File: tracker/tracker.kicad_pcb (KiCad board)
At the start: 2 copper layers, 26 parts, among them J1 USB_C_Receptacle_PowerOnly_6P, Q1 DMG9926UDM-7, U1 XIAO-ESP32-C6-SMD, U2 LIS3DH, U3 DW01A, U4 INA226AIDGSR, U5 TP4056-42-ESOP8

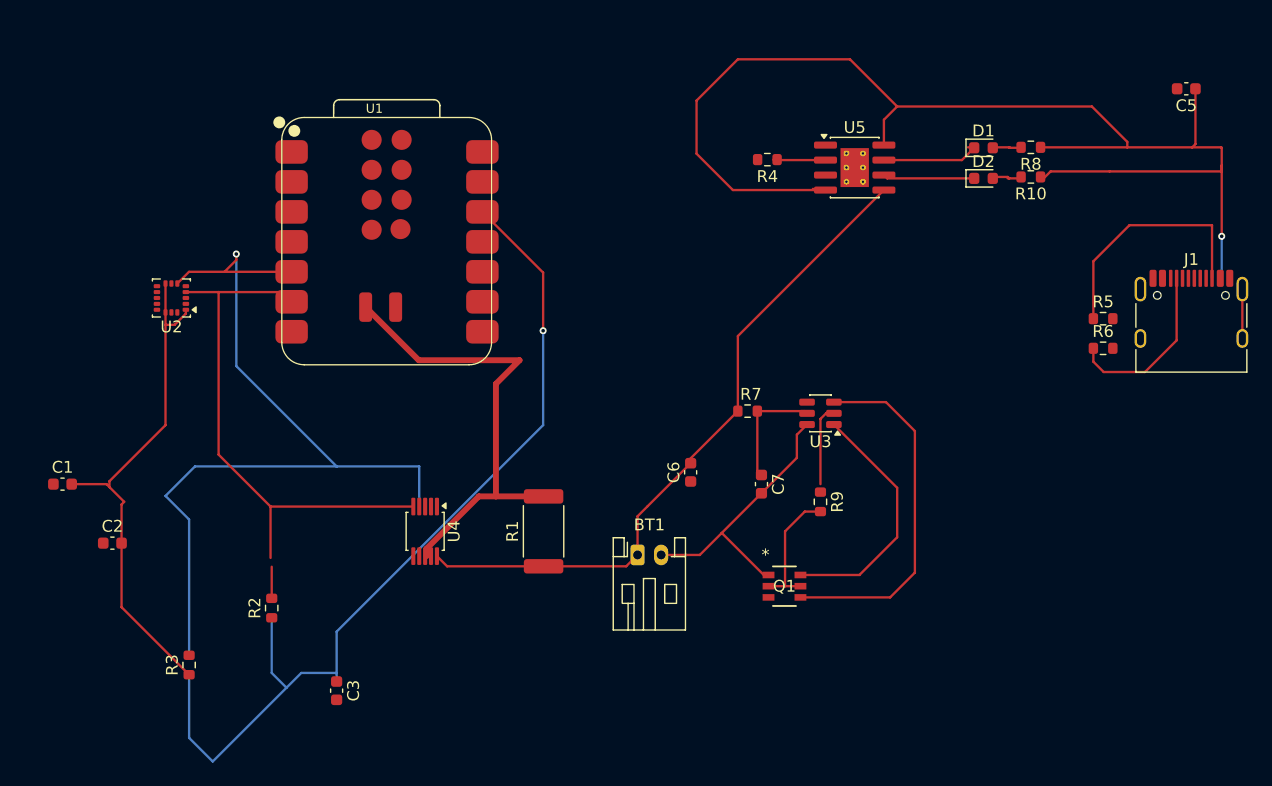
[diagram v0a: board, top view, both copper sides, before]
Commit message: working on ground
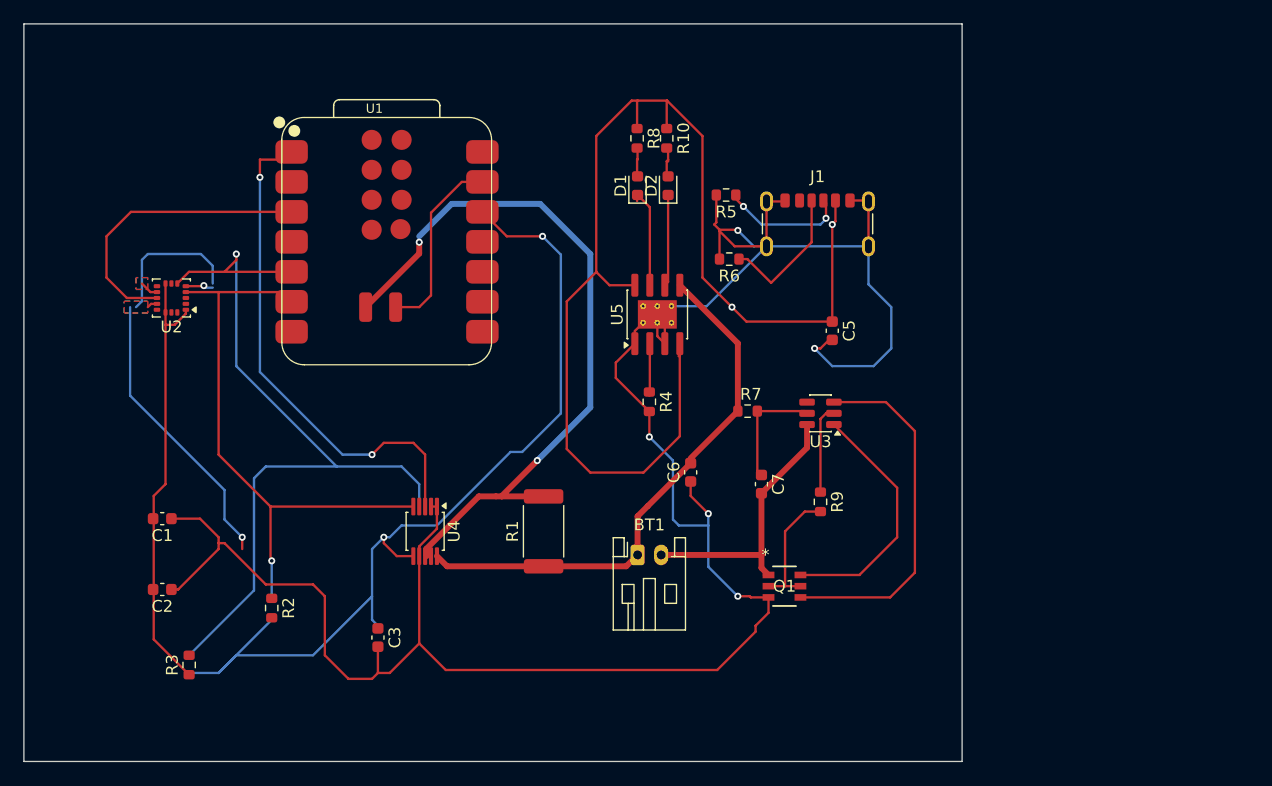
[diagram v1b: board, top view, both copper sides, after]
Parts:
- J1: footprint Connector_USB:USB_C_Receptacle_HRO_TYPE-C-31-M-12 -> Connector_USB:USB_C_Receptacle_GCT_USB4125-xx-x-0190_6P_TopMnt_Horizontal
- moved C5 36.3 mm to (158.0, 96.5), turned to -90 degrees
- moved R5 33.6 mm to (149.0, 85.0), turned to 180 degrees
- moved R8 33.4 mm to (141.5, 80.2), turned to -90 degrees
- moved J1 32.6 mm to (156.8, 88.5)
- moved R6 32.6 mm to (149.3, 90.4), turned to 180 degrees
- moved R10 31.0 mm to (144.0, 80.2), turned to -90 degrees
- moved D1 29.5 mm to (141.5, 84.2), turned to 90 degrees
- moved D2 26.7 mm to (144.1, 84.2), turned to 90 degrees
- moved R4 22.8 mm to (142.5, 102.5), turned to -90 degrees
- moved U5 20.8 mm to (143.2, 95.1), turned to 90 degrees
- moved C1 8.94 mm to (101.2, 112.4), turned to 180 degrees
- moved C2 5.77 mm to (101.2, 118.4), turned to 180 degrees
- moved C3 5.70 mm to (119.5, 122.5)
- turned R2 to -90 degrees
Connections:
- net -VSW renamed GND
- R2 pad 1: (no net) -> SCL
- R2 pad 2: (no net) -> 3v3
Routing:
- net GND: track 4.35 -> 221.2 mm, vias 0 -> 6
- net Net-(U1-D0): track 0.00 -> 43.1 mm, vias 0 -> 2
- net (no net): track 2.67 -> 36.8 mm, vias 0 -> 1
- net Net-(U1-D2): track 0.00 -> 25.0 mm
- net /Shunt_Output: track 39.7 -> 60.8 mm, vias 0 -> 2
- net /Charging_and_Battery/BAT+: track 57.3 -> 46.2 mm
- net Net-(J1-CC2): track 20.7 -> 10.7 mm, vias 0 -> 2
- net USB_VBUS: track 110.4 -> 103.5 mm, vias 1 -> 2
- net 3v3: track 120.7 -> 113.9 mm, vias 1 -> 2
- net SDA: track 73.4 -> 67.4 mm
- net SCL: track 45.8 -> 49.0 mm, vias 0 -> 1
- net Net-(J1-CC1): track 14.9 -> 12.0 mm
- net Net-(U3-CS): track 6.86 -> 7.53 mm
- added copper zone on B.Cu, net GND
- added copper zone on F.Cu, net GND
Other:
- board outline added: 79.5 x 62.5 mm
